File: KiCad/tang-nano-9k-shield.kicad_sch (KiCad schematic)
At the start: 0 parts

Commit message: Add files via upload
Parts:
- added BZ1: Buzzer, symbol Device:Buzzer
- added C10, C11, C14, C22, C4, C5, C9: 100nF, symbol Device:C_Small
- added C12, C13: 2.2nF, symbol Device:C_Small
- added C15, C2, C3, C8: 10uF, symbol Device:C_Small
- added C16, C17: 1uF, symbol Device:C_Small
- added C18, C19: 47pF, symbol Device:C_Small
- added C20, C21: 100uF, symbol Device:C_Small
- added C6, C7: 22uF, symbol Device:C_Small
- added D1: SS14, Diode_SMD:D_SMA, symbol Diode:SS14
- added D2: 1N4148W, Diode_SMD:D_SOD-123, symbol Diode:1N4148W
- added J1: Barrel_Jack, symbol Connector:Barrel_Jack
- added J2: AudioJack3, symbol Connector_Audio:AudioJack3
- added L1: 3.3uH, symbol Device:L_Small
- added Q1: SS8050, Package_TO_SOT_SMD:SOT-23, symbol Transistor_BJT:SS8050
- added R1, R2, R3, R4: 4K7, symbol Device:R_Small
- added R10, R11, R5, R9: 330R, symbol Device:R_Small
- added R12, R13: 47R, symbol Device:R_Small
- added R14, R15, R16, R17, R21, R6, R8: 10K, symbol Device:R_Small
- added R18: 1K, symbol Device:R_Small
- added R19, R20: 20K, symbol Device:R_Small
- added R7: 54K9, symbol Device:R_Small
- added U1: Tang Nano 9K, symbol TangNano9K:Tang-Nano-9K
- added U2: (no value), symbol TangNano9K:Dual-PS/2
- added U3: TPS563201DDCR, TPS563201DDCR:SOT95P280X110-6N, symbol TPS563201DDCR:TPS563201DDCR
- added U4: AMS1117-3.3, Package_TO_SOT_SMD:SOT-223-3_TabPin2, symbol Regulator_Linear:AMS1117-3.3
- added U5: PT8211, PT8211:SOP8-6.0-4.9X3.9, symbol PT8211:PT8211
- added U6: LMV358, symbol Amplifier_Operational:LMV358
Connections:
- new net: R5.1, U2.1
- new net: C15.1, R14.2, R15.1, U6.3 (+), U6.5 (+)
- new net: C18.1, R17.2, R19.1, U6.6 (-)
- new net: C18.2, C21.1, R19.2, U6.7
- new net: C2.1, C3.1, C4.1, D1.1 (K), R6.2, U3.3 (VIN)
- new net: R13.1, U5.6 (LCH)
- new net: R6.1, U3.5 (EN)
- new net: R10.1, U2.7
- new net: C16.2, R16.1
- new net: C19.1, R16.2, R20.1, U6.2 (-)
- new net: R9.1, U2.11
- new net: R11.1, U2.5
- new net: Q1.1 (B), R18.2
- new net: C5.1, L1.1, U3.2 (SW)
- new net: D1.2 (A), J1.1
- new net: C5.2, U3.6 (VBST)
- new net: C17.2, R17.1
- new net: C19.2, C20.1, R20.2, U6.1
- new net: C21.2, J2.R
- new net: BZ1.2 (-), D2.2 (A), Q1.3 (C)
- new net: R12.1, U5.8 (RCH)
- new net: R7.2, R8.1, U3.4 (VFB)
- new net: C20.2, J2.T
- new net 3V3: C8.1, C9.1, R1.1, R2.1, R3.1, R4.1, U4.2 (VO)
- new net 5V: BZ1.1 (+), C10.1, C11.1, C14.1, C22.1, C6.1, C7.1, D2.1 (K), L1.2, R14.1, R7.1, U1.5V, U2.10, U2.4, U4.3 (VI), U5.5 (VDD), U6.8 (V+)
- new net BCK: U1.51 (IOR17B), U5.1 (BCK)
- new net BUZ: R18.1, R21.2, U1.38 (IOB31B)
- new net DIN: U1.54 (IOR15A), U5.3 (DIN)
- new net GND: C10.2, C11.2, C12.2, C13.2, C14.2, C15.2, C2.2, C22.2, C3.2, C4.2, C6.2, C7.2, C8.2, C9.2, J1.2, J2.S, Q1.2 (E), R15.2, R21.1, R8.2, U1.GND, U2.3, U2.9, U2.MP, U3.1 (GND), U4.1 (GND), U5.4 (GND), U6.4 (V-)
- new net LCH: C13.1, C16.1, R13.2
- new net PS/2_CLK1: R1.2, R11.2, U1.71 (IOT41A)
- new net PS/2_CLK2: R3.2, R9.2, U1.48 (IOR24B)
- new net PS/2_DAT1: R2.2, R5.2, U1.70 (IOT41B)
- new net PS/2_DAT2: R10.2, R4.2, U1.49 (IOR24A)
- new net RCH: C12.1, C17.1, R12.2
- new net WS: U1.53 (IOR15B), U5.2 (WS)
- no-connect marks 0 -> 5
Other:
- note added: "AUDIO"
- note added: "Left"
- note added: "POWER"
- note added: "PS/2"
- note added: "Right"

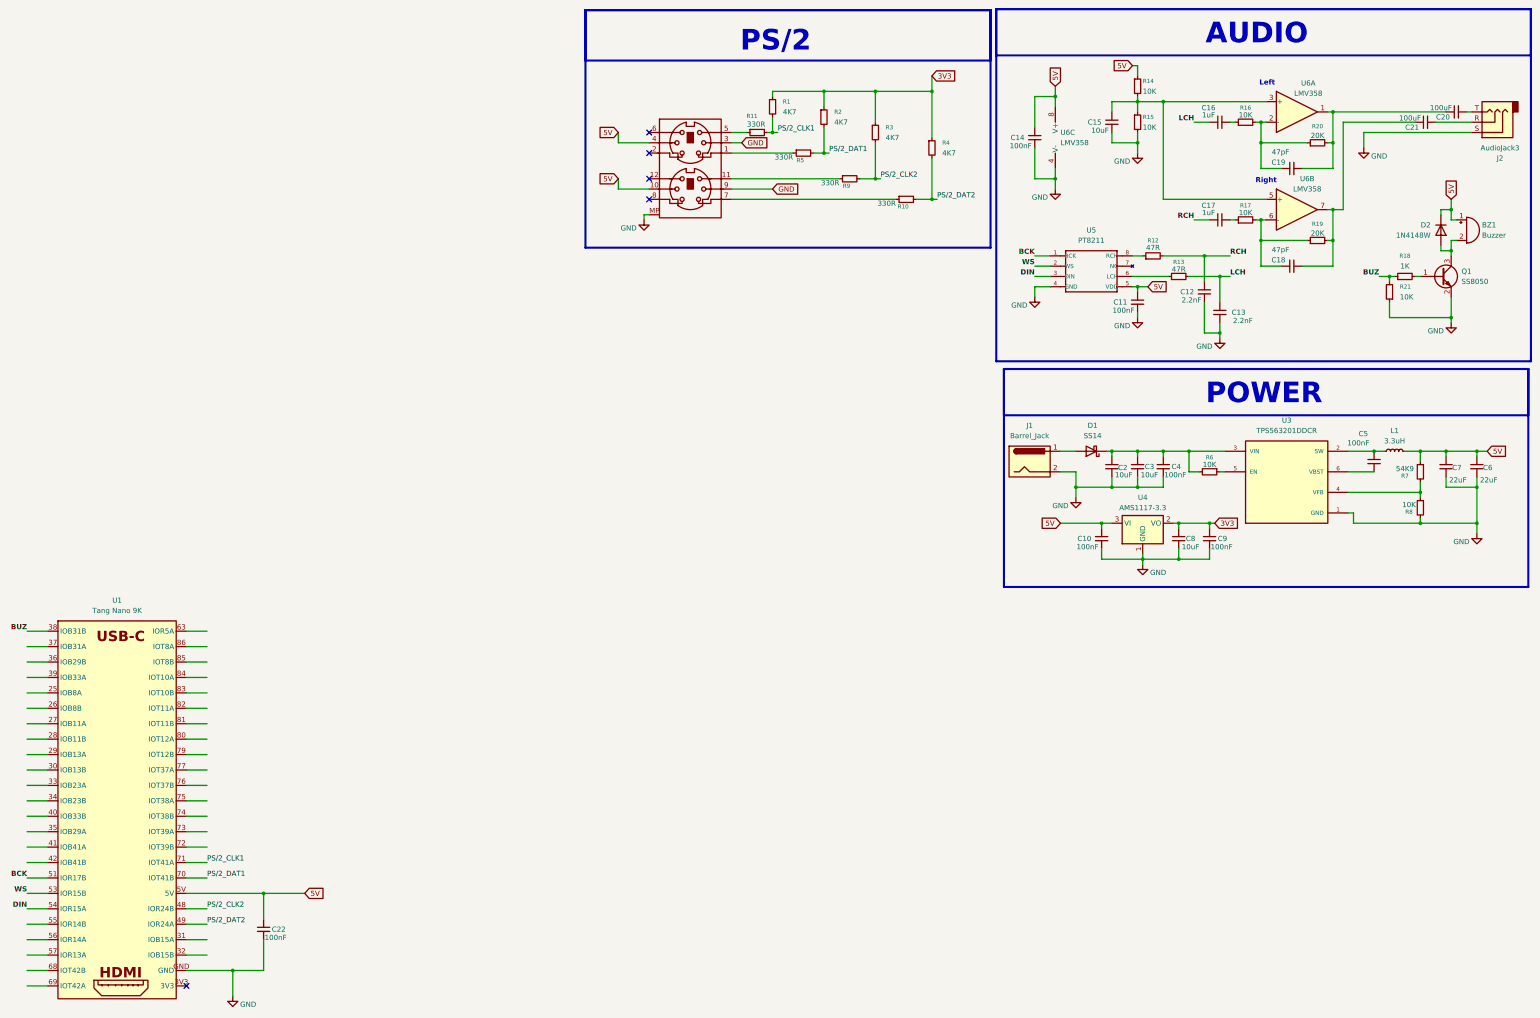
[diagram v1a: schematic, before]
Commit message: Add files via upload
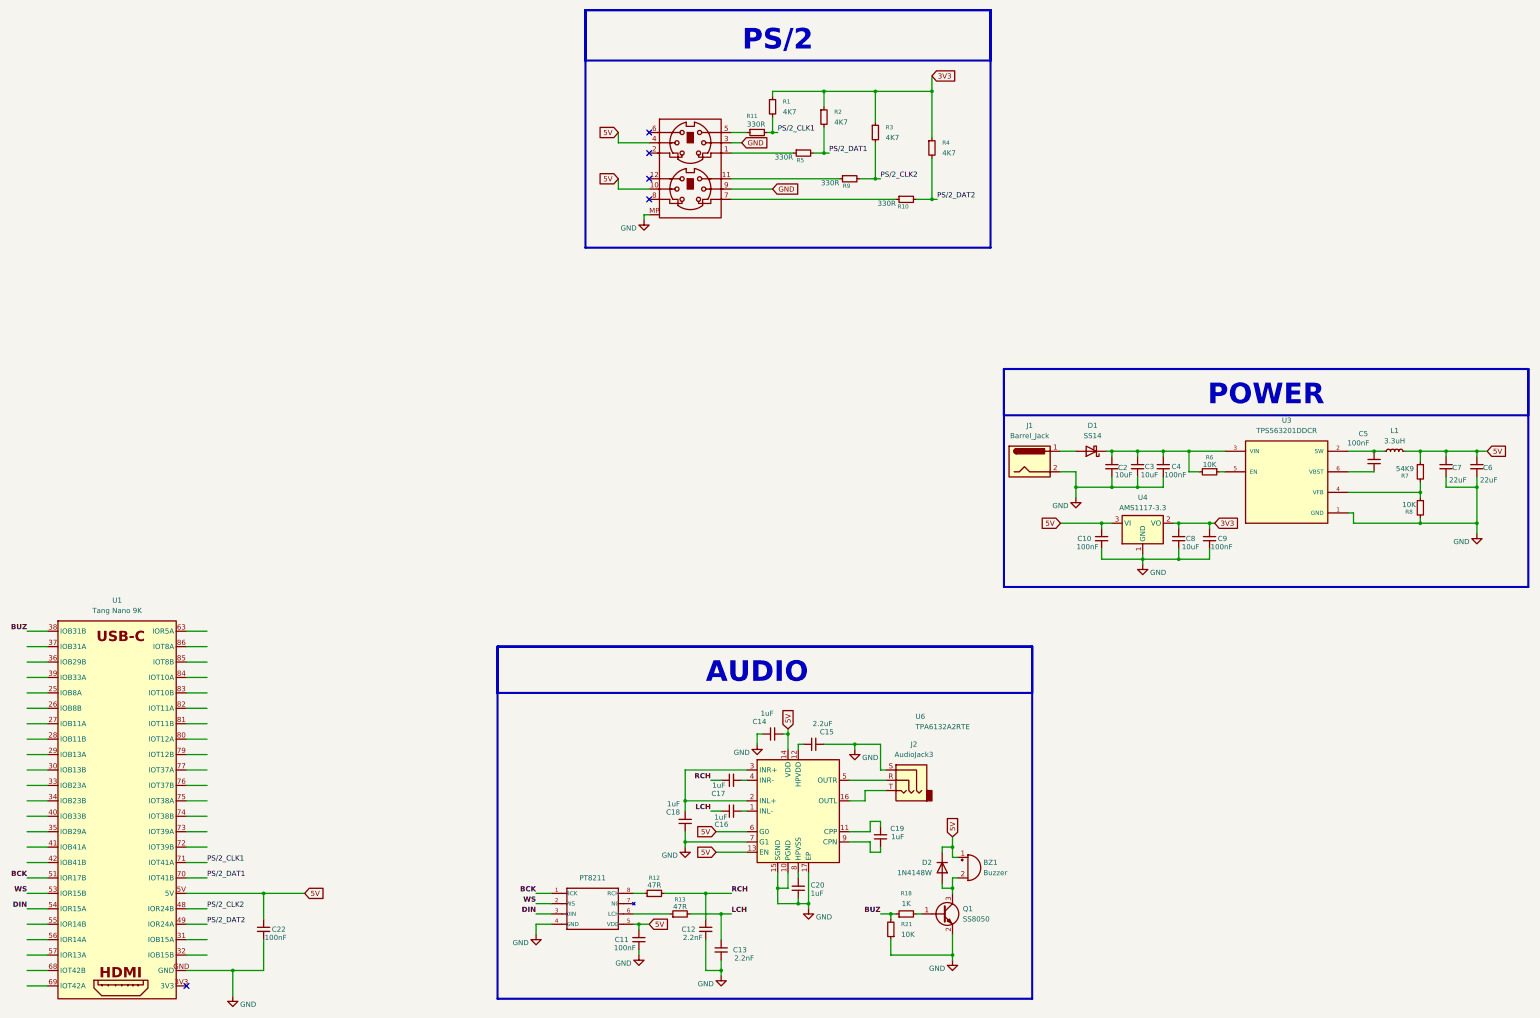
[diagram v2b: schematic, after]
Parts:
- removed C21: 100uF, symbol Device:C_Small
- removed R14, R15, R16, R17: 10K, symbol Device:R_Small
- removed R19, R20: 20K, symbol Device:R_Small
- removed U6: LMV358, symbol Amplifier_Operational:LMV358
- added U6: TPA6132A2RTE, Package_DFN_QFN:WQFN-16-1EP_3x3mm_P0.5mm_EP1.6x1.6mm_ThermalVias, symbol Amplifier_Audio:TPA6132A2RTE
- C14: value 100nF -> 1uF
- C15: value 10uF -> 2.2uF
- C18, C19: value 47pF -> 1uF
- C20: value 100uF -> 1uF
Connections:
- net 5V: now also C14.2, U6.13 (EN), U6.14 (VDD), U6.6 (G0); no longer C14.1
- net GND: now also C14.1, C15.1, C18.1, C20.1, U6.10 (PGND), U6.15 (SGND), U6.17 (EP), U6.7 (G1); no longer C14.2, C15.2
- net at C18.2: now also U6.2 (INL+), U6.3 (INR+)
- net at C16.2: now also U6.1 (INL-)
- net at C19.1: now also U6.9 (CPN)
- net at C17.2: now also U6.4 (INR-)
- net at C19.2: now also U6.11 (CPP); no longer C20.1
- net at J2.R: now also U6.5 (OUTR)
- net at J2.T: now also U6.16 (OUTL); no longer C20.2
- new net: C20.2, U6.8 (HPVSS)
- new net: C15.2, U6.12 (HPVDD)
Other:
- note removed: "Left"
- note removed: "Right"
- moved on the sheet: BZ1, C11, C12, C13, D2, J2, Q1, R12, R13, R18, R21
